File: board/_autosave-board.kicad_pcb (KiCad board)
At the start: 2 copper layers, 66.1 x 100.8 mm, 27 parts, among them J1 port attiny, J10 BMS Bat +, J11 BMS Bat gnd, J12 BMS out -, J13 BMS in +5v, J14 BMS in gnd, J15_C189893 BMS led charge ok, J16 Mp3 D1 led marche ok, J17 Haut parleur, J18 Batterie + et -, J19 BMS in + et -, J2 alim attiny, J20 BMS led charge ok, J21 Vers bouton vol - et next, J22_C189893 Mp3 D1 led marche ok, J23-C189893 alim +5 gnd, J3 alim mp3, J4 hp mp3, J5 vol - et next +, J6 step up out, J7 step up in +, J8 step up in -, J9 BMS out +

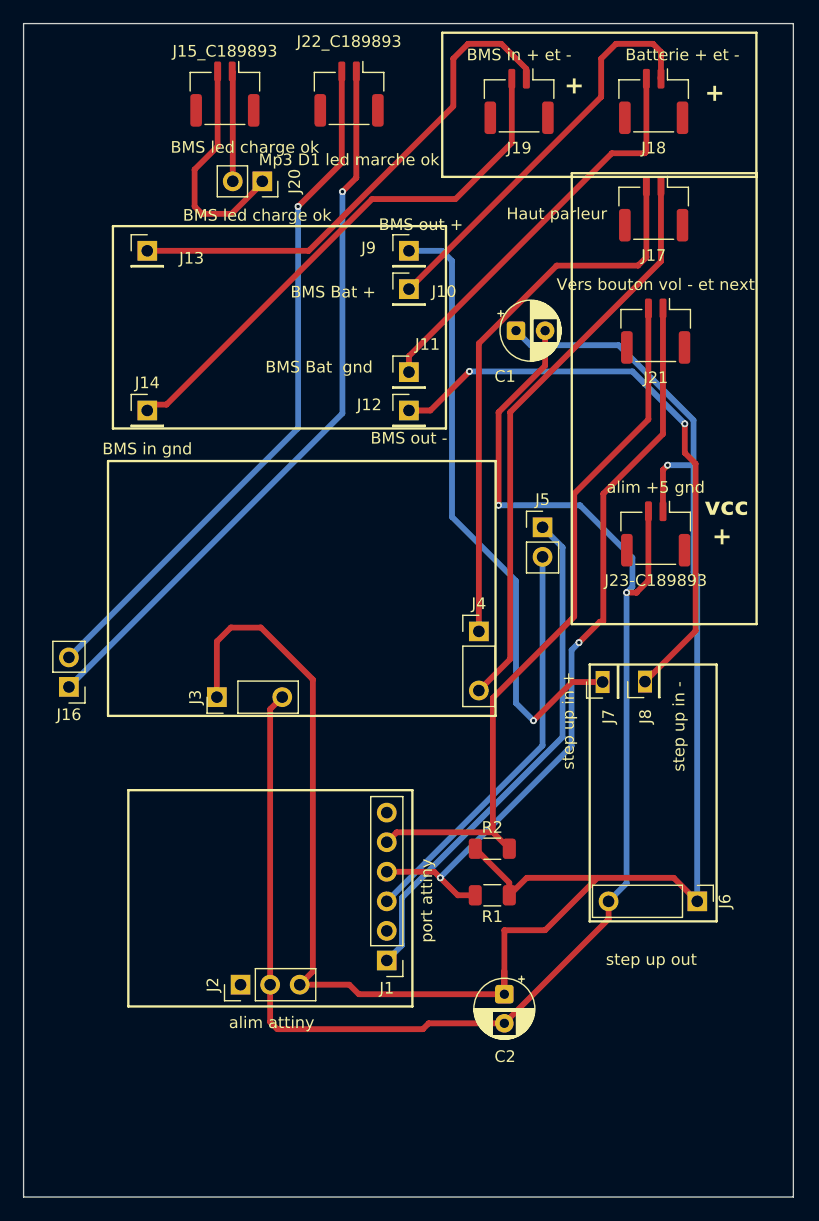
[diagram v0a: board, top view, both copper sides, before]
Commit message: mise a jour pcb
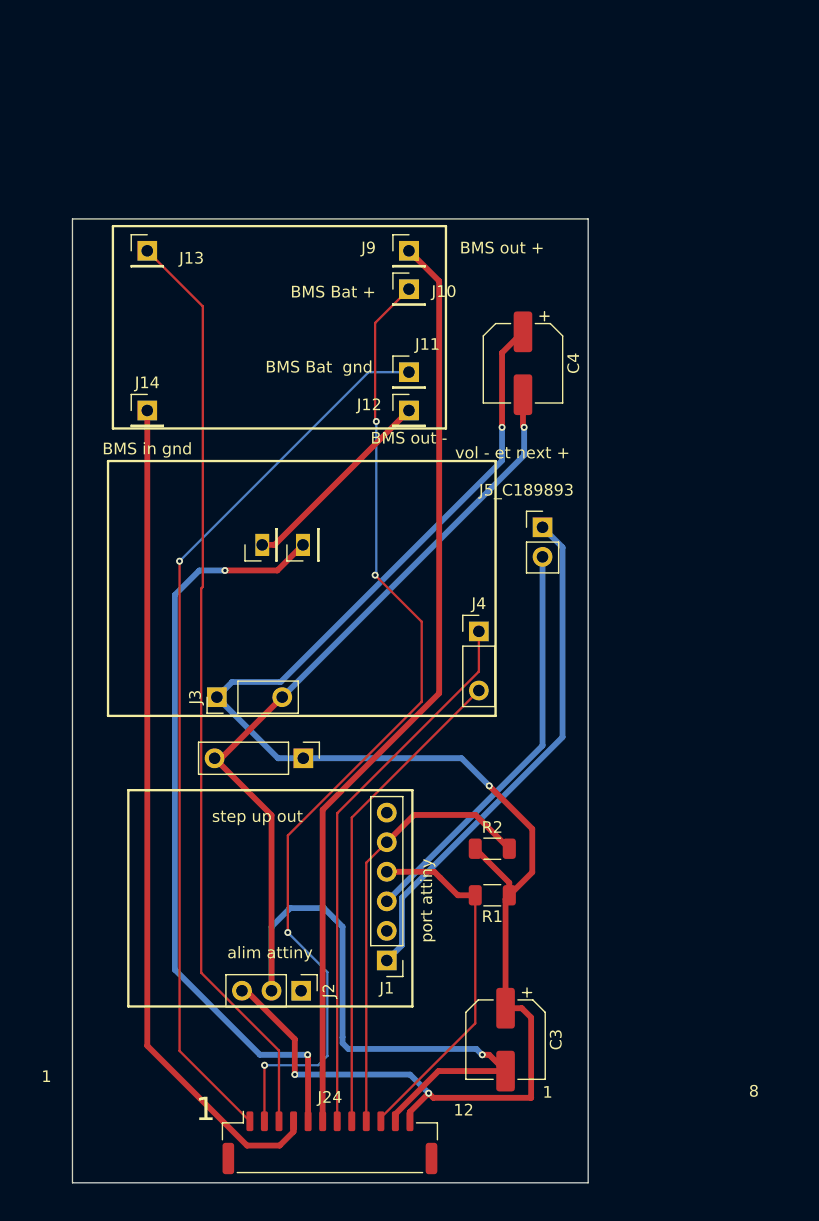
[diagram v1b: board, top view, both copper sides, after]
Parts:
- removed C1, C2: C, Capacitor_THT:CP_Radial_D5.0mm_P2.50mm
- removed J15_C189893: BMS led charge ok, Connector_JST:JST_GH_BM02B-GHS-TBT_1x02-1MP_P1.25mm_Vertical
- removed J16: Mp3 D1 led marche ok, Connector_PinHeader_2.54mm:PinHeader_1x02_P2.54mm_Vertical
- removed J17: Haut parleur, Connector_JST:JST_GH_BM02B-GHS-TBT_1x02-1MP_P1.25mm_Vertical
- removed J18: Batterie + et -, Connector_JST:JST_GH_BM02B-GHS-TBT_1x02-1MP_P1.25mm_Vertical
- removed J19: BMS in + et -, Connector_JST:JST_GH_BM02B-GHS-TBT_1x02-1MP_P1.25mm_Vertical
- removed J20: BMS led charge ok, Connector_PinSocket_2.54mm:PinSocket_1x02_P2.54mm_Vertical
- removed J21: Vers bouton vol - et next, Connector_JST:JST_GH_BM02B-GHS-TBT_1x02-1MP_P1.25mm_Vertical
- removed J22_C189893: Mp3 D1 led marche ok, Connector_JST:JST_GH_BM02B-GHS-TBT_1x02-1MP_P1.25mm_Vertical
- removed J23-C189893: alim +5 gnd, Connector_JST:JST_GH_BM02B-GHS-TBT_1x02-1MP_P1.25mm_Vertical
- added C3: C_C22388053, Capacitor_SMD:CP_Elec_6.3x7.7, F.Cu at (99.1, 108.4)
- added C4: C_C22388053, Capacitor_SMD:CP_Elec_6.3x7.7, F.Cu at (100.6, 50.3)
- added J24: port 3-C265421, Connector_JST:JST_GH_SM12B-GHS-TB_1x12-1MP_P1.25mm_Horizontal, F.Cu at (84.0, 117.3)
- J7: value step up in + -> +
- J8: value step up in - -> -
- R1, R2: value 4.7kΩ _C2907499 -> 4.7kΩ _C17936
- moved J6 36.0 mm to (81.7, 84.2)
- moved J8 34.9 mm to (78.1, 65.9)
- moved J7 28.3 mm to (81.7, 65.9)
- moved J2 5.23 mm to (81.5, 104.2), turned to -90 degrees
- renumbered J5 to J5_C189893
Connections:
- J7 pad 1: Net-(J7-Pin_1) -> Net-(J23-Pin_2)
- J9 pad 1: Net-(J7-Pin_1) -> Net-(J23-Pin_1)
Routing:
- net Net-(J23-Pin_1): track 0.00 -> 80.7 mm
- net Net-(J23-Pin_2): track 0.00 -> 66.5 mm, vias 0 -> 2
- net Net-(J16-Pin_1): track 63.1 -> 0.00 mm, vias 1 -> 0
- net Net-(J16-Pin_2): track 60.0 -> 0.00 mm, vias 1 -> 0
- net Net-(J7-Pin_1): track 53.8 -> 0.00 mm, vias 1 -> 0
- net Net-(J10-Pin_1): track 35.0 -> 85.5 mm, vias 0 -> 4
- net Net-(J11-Pin_1): track 35.3 -> 77.2 mm, vias 0 -> 1
- net Net-(J13-Pin_1): track 44.1 -> 79.6 mm
- net Net-(J1-Pin_4): track 65.4 -> 31.2 mm, vias 2 -> 0
- net Net-(J12-Pin_1): track 51.3 -> 17.4 mm, vias 2 -> 0
- net Net-(J14-Pin_1): track 46.3 -> 72.8 mm
- net VCC: track 166.4 -> 141.0 mm, vias 1 -> 4
- net Net-(J1-Pin_5): track 62.0 -> 38.1 mm
- net Net-(J15_C189893-Pin_2): track 19.8 -> 0.00 mm
- net GND: track 131.8 -> 114.7 mm
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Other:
- board size 66.1 x 100.8 mm -> 44.3 x 82.8 mm
- board text added: "1"
- board text added: "1 : bat + 2 : bat gnd 3 : BMS in + 4 : BMS in gnd 5 : on/off 6 : on/off 7 : HP + 8 : HP - 9 : bouton VOL - 10 : bouton NEXT 11 : vcc 12 : gnd"
- board text added: "12"
- board text added: "8"
- board text removed: "+"
- board text removed: "vcc"
